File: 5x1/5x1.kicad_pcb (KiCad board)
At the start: 2 copper layers, 94 x 19.1 mm, 7 parts, among them J1 Conn_01x10_Male, U1 Elite-C

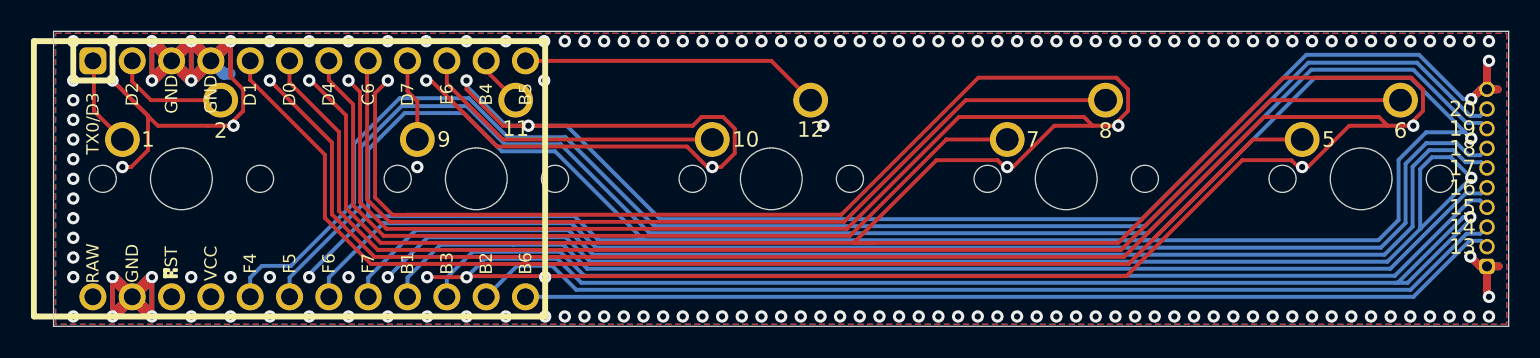
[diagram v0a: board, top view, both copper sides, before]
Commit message: 5trange dot as built
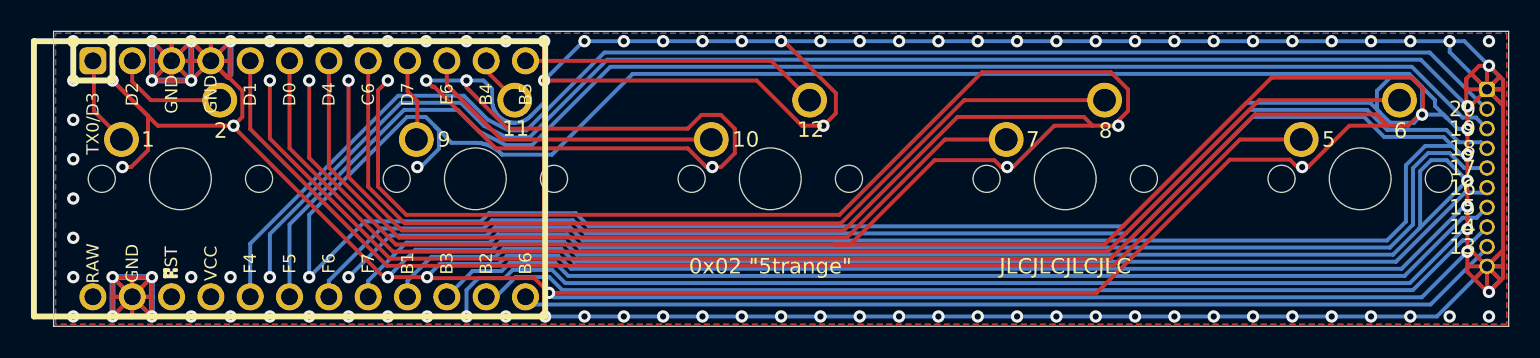
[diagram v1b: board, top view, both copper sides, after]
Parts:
- removed J1: Conn_01x10_Male, Connector_PinHeader_1.27mm:PinHeader_1x10_P1.27mm_Vertical
- removed MX_0: MX-NoLED, MX_Only:MXOnly-1U-NoLED
- added J_0: Conn_01x10_Male, Connector_PinHeader_1.27mm:PinHeader_1x10_P1.27mm_Vertical, F.Cu at (92.6, 3.75)
- added MX_5: MX-NoLED, MX_Only:MXOnly-1U-NoLED, F.Cu at (84.4, 9.53)
- moved MX_1 19.1 mm to (8.19, 9.53)
- moved MX_3 19.1 mm to (46.3, 9.53)
- moved MX_4 19.1 mm to (65.3, 9.53)
- moved MX_2 19.1 mm to (27.2, 9.53)
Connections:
- MX_1 pad 1: C1 -> C0
- MX_1 pad 2: R1 -> R0
- MX_2 pad 1: C2 -> C1
- MX_2 pad 2: R2 -> R1
- MX_3 pad 1: C3 -> C2
- MX_3 pad 2: R3 -> R2
- MX_4 pad 1: C4 -> C3
- MX_4 pad 2: R4 -> R3
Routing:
- net GND: track 899.4 -> 1483.7 mm, vias 171 -> 118
- net Net-(J_0-Pad2): track 97.6 -> 91.7 mm
- net Net-(J_0-Pad3): track 94.8 -> 89.6 mm
- net Net-(J_0-Pad7): track 72.0 -> 70.3 mm
- net Net-(J_0-Pad4): track 83.7 -> 82.1 mm
- net Net-(J_0-Pad5): track 81.0 -> 80.0 mm
- net Net-(J_0-Pad6): track 74.7 -> 74.0 mm
- net Net-(J_0-Pad8): track 67.8 -> 67.3 mm
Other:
- net class Default: clearance 0.2 -> 0.2032; trace_width 0.25 -> 0.254
- rule trace_clearance: 0.2 -> 0.2032
- rule trace_min: 0.2032 -> 0.254
- board text added: "0x02 "5trange""
- board text added: "JLCJLCJLCJLC"
